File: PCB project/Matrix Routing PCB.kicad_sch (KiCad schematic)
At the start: 6 parts, among them J1 53261-0471, J2 JST_PH_S4B-PH-SM4-TB, J3 ESQ-105-23-T-D, J4 TSM-102-01-L-DH-A, J5 USB-A-S-X-X-SM2-R, U1 FT232RL

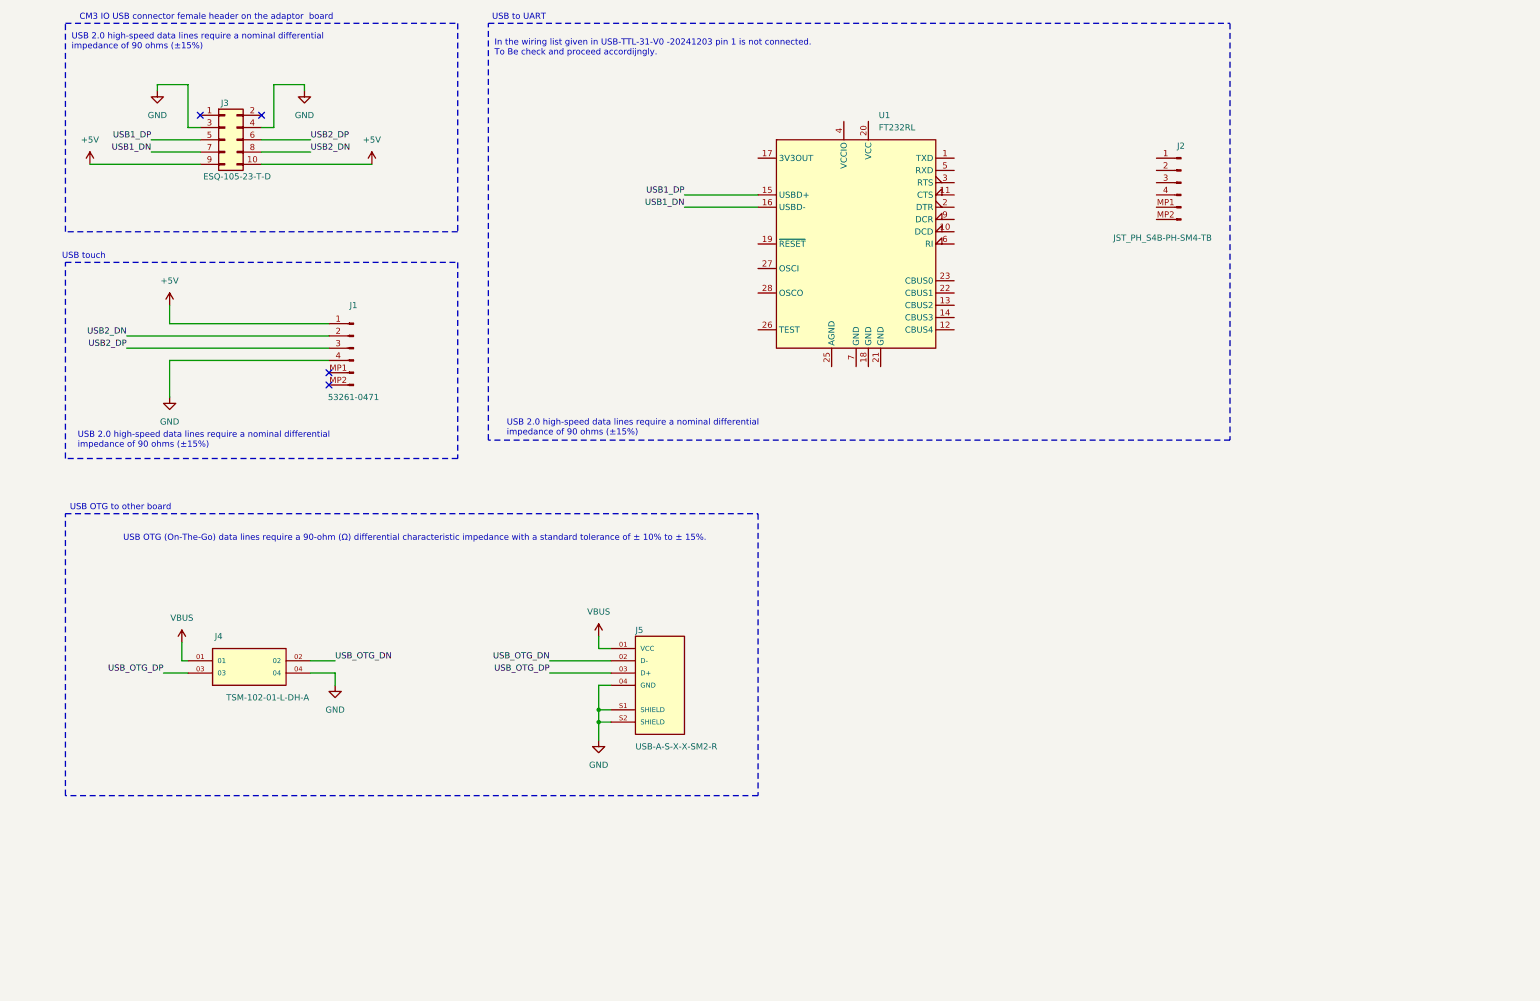
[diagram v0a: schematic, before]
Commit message: Schematic finish
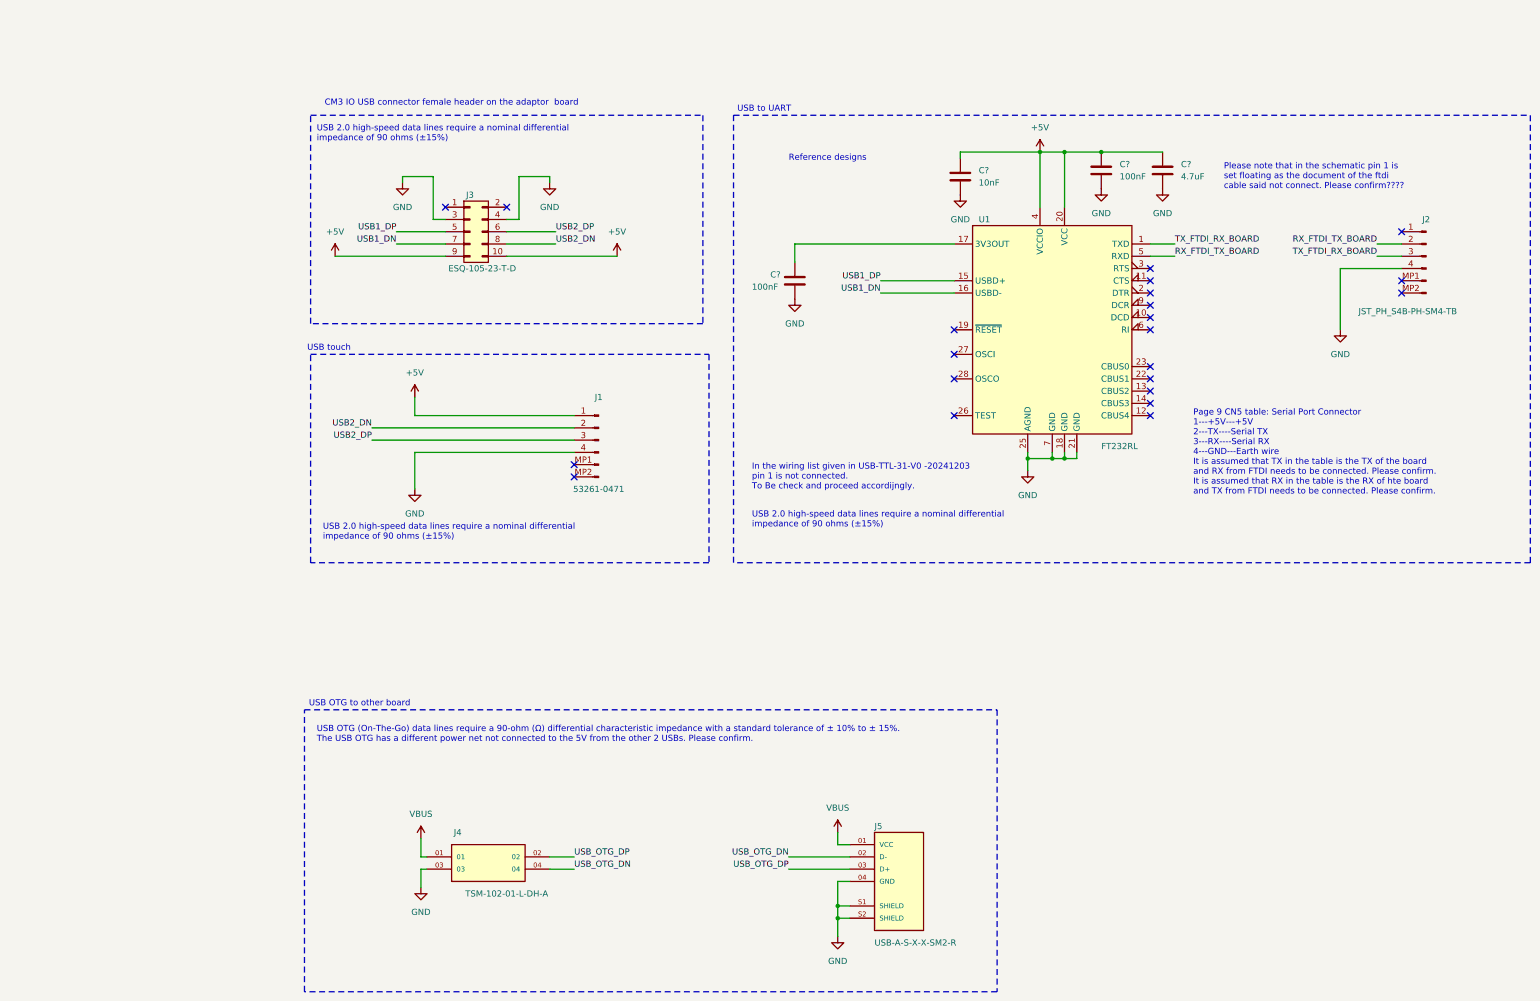
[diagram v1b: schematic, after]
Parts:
- added C?: 4.7uF, symbol Device:C
- added C? (x2): 100nF, symbol Device:C
- added C?: 10nF, symbol Device:C
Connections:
- net +5V: now also U1.20 (VCC), U1.4 (VCCIO), C?.1, C?.1, C?.1
- net GND: now also J2.4 (Pin_4), J4.03, U1.18 (GND), U1.21 (GND), U1.25 (AGND), U1.7 (GND), C?.2, C?.2, C?.2, C?.2; no longer J4.04
- net USB_OTG_DN: now also J4.04; no longer J4.02
- net USB_OTG_DP: now also J4.02; no longer J4.03
- net RX_FTDI_TX_BOARD: now reaches J2.2 (Pin_2)
- net RX_FTDI_TX_BOARD: now also U1.5 (RXD)
- net TX_FTDI_RX_BOARD: now reaches J2.3 (Pin_3)
- net TX_FTDI_RX_BOARD: now also U1.1 (TXD)
- net at U1.17 (3V3OUT): now also C?.1
- no-connect marks 4 -> 22
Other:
- note added: "Page 9 CN5 table: Serial Port Connector 1---+5V---+5V 2---TX----Serial TX 3---RX----Serial RX 4---GND---Earth wire It is assumed that TX in the table is the TX of the board and RX from FTDI needs to be connected. Please confirm. It is assumed that RX in the table is the RX of hte board and TX from FTDI needs to be connected. Please confirm."
- note added: "Please note that in the schematic pin 1 is set floating as the document of the ftdi cable said not connect. Please confirm????"
- note added: "Reference designs"
- note added: "USB OTG (On-The-Go) data lines require a 90-ohm (Ω) differential characteristic impedance with a standard tolerance of ± 10% to ± 15%. The USB OTG has a different power net not connected to the 5V from the other 2 USBs. Please confirm."
- note removed: "USB OTG (On-The-Go) data lines require a 90-ohm (Ω) differential characteristic impedance with a standard tolerance of ± 10% to ± 15%."
- title: (none) -> Matrix
- moved on the sheet: J1, J2, J3, J4, J5, U1
